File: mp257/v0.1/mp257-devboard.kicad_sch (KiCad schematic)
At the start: 39 parts, among them CON1 microSDCon_SMT_104031-0811, J1 Pins_02x40_P0.4mm_W3.0mm_SMT, J2 Pins_02x40_P0.4mm_W3.0mm_SMT, J3 USB-C_Receptacle_Molex_217179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, J4 Pins_02x04_RightAngle_P2.54mm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, J5 Conn_01x02, J6 Pins_02x05_P1.27mm_SMT, U1 STM32MP257FAK3, U3 USBLC6-2SC6, U5 NORFLASH_W25Q128JV, X2 40MHz_6.8pF_2x1.6mm

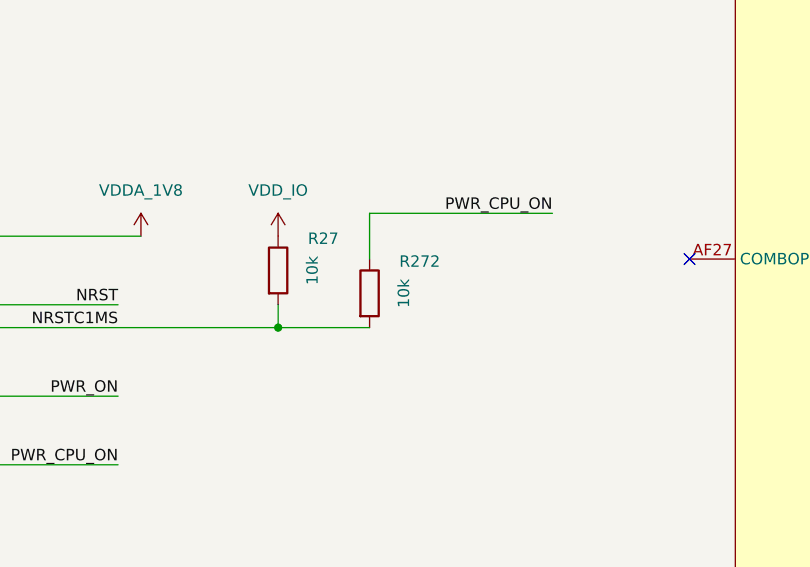
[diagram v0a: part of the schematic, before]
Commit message: WIP
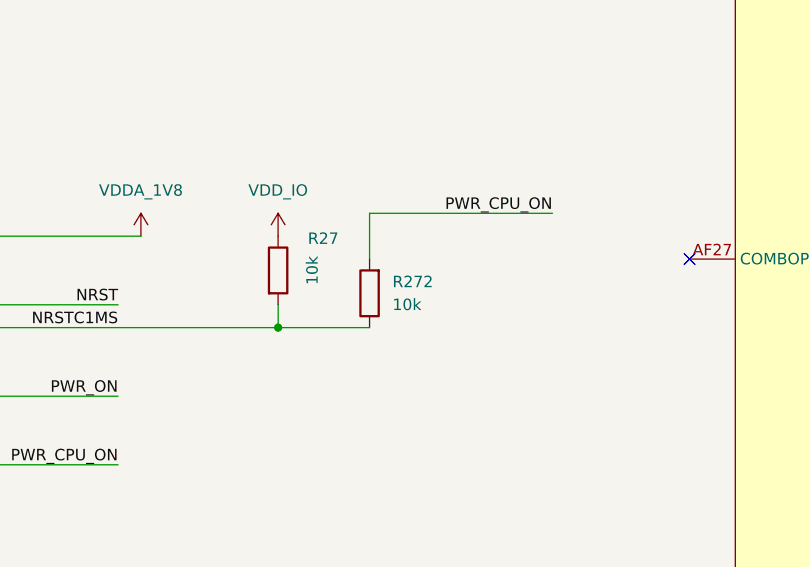
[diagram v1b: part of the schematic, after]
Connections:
- net NRSTC1MS: now also R272.1; no longer R272.2
- net PWR_CPU_ON: now also R272.2; no longer R272.1
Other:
- moved on the sheet: R272
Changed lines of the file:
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@@
 	(symbol
 		(lib_id "4ms_Resistor_0402:10k_0402")
-		(at 153.67 485.14 0)
+		(at 153.67 485.14 180)
 		(unit 1)
 		(exclude_from_sim no)
@@
 		(on_board yes)
 		(dnp no)
+		(fields_autoplaced yes)
 		(property "Reference" "R272"
-			(at 156.972 482.346 0)
+			(at 156.21 483.8699 0)
 			(effects
 				(font
 					(size 1.27 1.27)
 				)
-				(justify left bottom)
+				(justify right)
 			)
 		)
 		(property "Value" "10k_0402"
-			(at 151.13 485.14 90)
+			(at 156.21 485.14 90)
 			(effects
 				(font
@@
 		)
 		(property "Footprint" "4ms_Resistor:R_0402"
-			(at 151.13 498.094 0)
+			(at 156.21 472.186 0)
 			(effects
 				(font
@@
 		)
 		(property "Specifications" "10k, 1%, 1/16W, 0402"
-			(at 151.13 492.76 0)
+			(at 156.21 477.52 0)
 			(effects
 				(font
@@
 		)
 		(property "Manufacturer" "Yageo"
-			(at 151.13 494.538 0)
+			(at 156.21 475.742 0)
 			(effects
 				(font
@@
 		)
 		(property "Part Number" "RC0402FR-0710KL"
-			(at 151.13 496.316 0)
+			(at 156.21 473.964 0)
 			(effects
 				(font
@@
 		)
 		(property "Display" "10k"
-			(at 157.48 485.14 90)
+			(at 156.21 486.4099 0)
 			(effects
 				(font
 					(size 1.27 1.27)
 				)
+				(justify right)
 			)
 		)
 		(property "JLCPCB ID" "C60490"
-			(at 151.13 499.872 0)
+			(at 156.21 470.408 0)
 			(effects
 				(font
@@
 		)
 		(property "Production Stage" "A"
-			(at 151.13 501.65 0)
+			(at 156.21 468.63 0)
 			(effects
 				(font
